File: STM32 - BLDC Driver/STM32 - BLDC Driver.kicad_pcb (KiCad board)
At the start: 2 copper layers, 15 parts, among them J1 Conn_01x02_Pin, J4 TC2050, U1 STM32F411CEUx, U2 LM2596S-3.3, U6 LD1117S33TR_SOT223, U7 LM66100DCK, U8 LM66100DCK

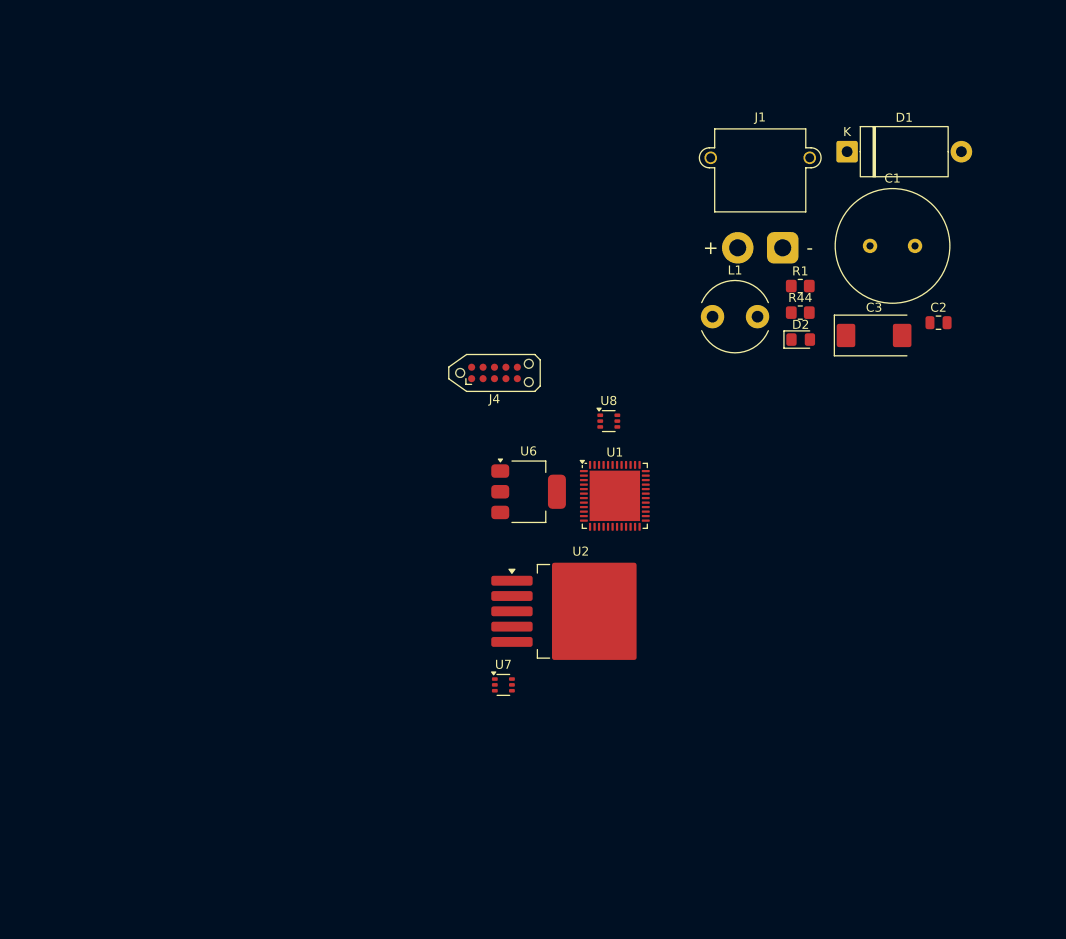
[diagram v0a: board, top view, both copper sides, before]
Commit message: As manufactured.
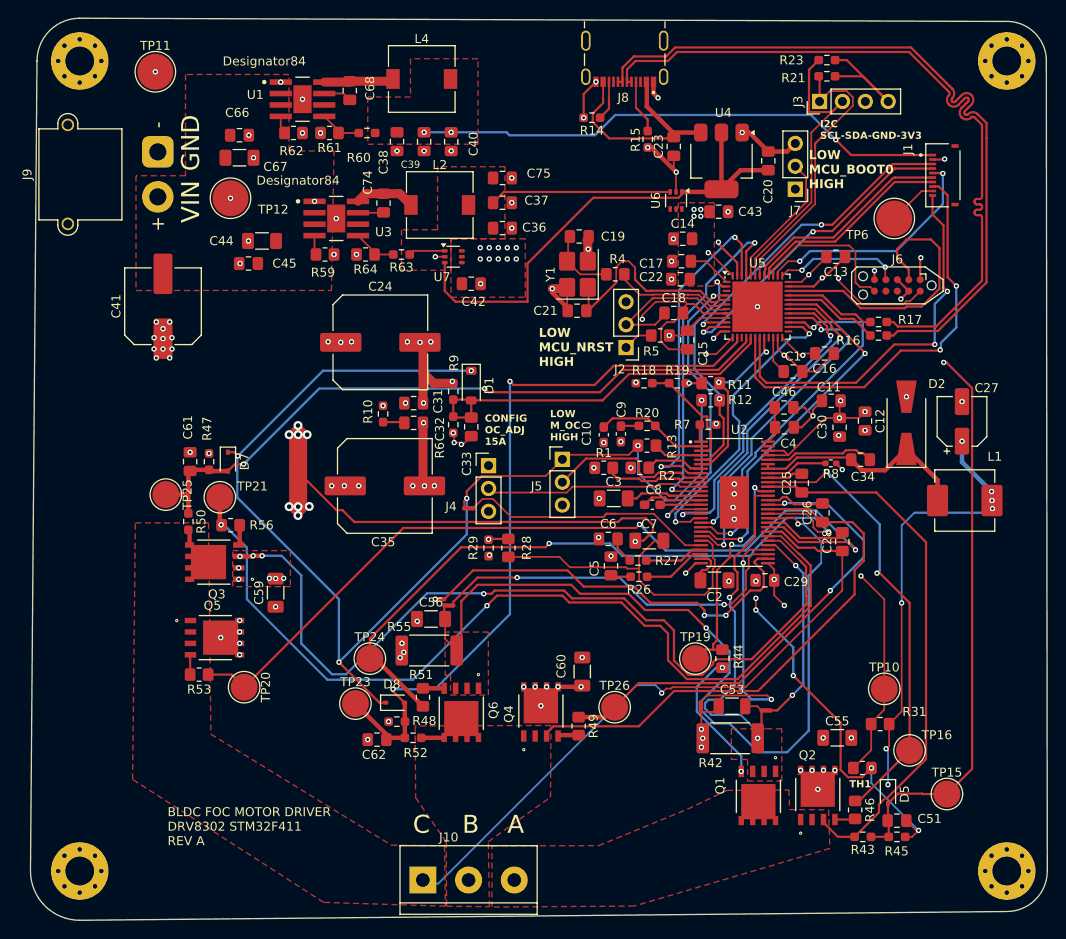
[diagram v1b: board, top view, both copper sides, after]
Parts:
- removed U8: LM66100DCK, Package_TO_SOT_SMD:SOT-363_SC-70-6
- added C10: 120p (C107035), Capacitor_SMD:C_0603_1608Metric_Pad1.08x0.95mm_HandSolder, F.Cu at (79.2, 61.5)
- added C11: 4.7u low esr (C1779), Capacitor_SMD:C_0805_2012Metric_Pad1.18x1.45mm_HandSolder, F.Cu at (104.5, 57.8)
- added C12: 4.7u low esr (C1779), Capacitor_SMD:C_0805_2012Metric_Pad1.18x1.45mm_HandSolder, F.Cu at (108.2, 60.0)
- added C13: 100nF 50V (C28233), Capacitor_SMD:C_0805_2012Metric_Pad1.18x1.45mm_HandSolder, F.Cu at (105.0, 41.8)
- added C14: 100nF 50V (C28233), Capacitor_SMD:C_0805_2012Metric_Pad1.18x1.45mm_HandSolder, F.Cu at (88.0, 39.8)
- added C15: 100nF 50V (C28233), Capacitor_SMD:C_0805_2012Metric_Pad1.18x1.45mm_HandSolder, F.Cu at (88.5, 51.0)
- added C16: 100nF 50V (C28233), Capacitor_SMD:C_0805_2012Metric_Pad1.18x1.45mm_HandSolder, F.Cu at (103.8, 52.5)
- added C17: 2.2u (C5448893), Capacitor_SMD:C_0805_2012Metric_Pad1.18x1.45mm_HandSolder, F.Cu at (87.9, 42.2)
- added C18: 100nF 50V (C28233), Capacitor_SMD:C_0805_2012Metric_Pad1.18x1.45mm_HandSolder, F.Cu at (87.0, 48.0)
- added C19: 100nF 50V (C28233), Capacitor_SMD:C_0805_2012Metric_Pad1.18x1.45mm_HandSolder, F.Cu at (76.5, 39.5)
- added C20: 10uF (C15850), Capacitor_SMD:C_0805_2012Metric_Pad1.18x1.45mm_HandSolder, F.Cu at (97.5, 31.1)
- added C21: 100nF 50V (C28233), Capacitor_SMD:C_0805_2012Metric_Pad1.18x1.45mm_HandSolder, F.Cu at (76.2, 47.8)
- added C22: 100nF 50V (C28233), Capacitor_SMD:C_0805_2012Metric_Pad1.18x1.45mm_HandSolder, F.Cu at (87.8, 44.2)
- added C23: 100nF 50V (C28233), Capacitor_SMD:C_0805_2012Metric_Pad1.18x1.45mm_HandSolder, F.Cu at (87.0, 29.5)
- added C24: 220uF (C46550422), Capacitor_SMD:C_Elec_10x10.2, F.Cu at (54.4, 51.3)
- added C25: 0.1uF (C28233), Capacitor_SMD:C_0805_2012Metric_Pad1.18x1.45mm_HandSolder, F.Cu at (101.2, 66.9)
- added C26: 0.1uF (C28233), Capacitor_SMD:C_0805_2012Metric_Pad1.18x1.45mm_HandSolder, F.Cu at (103.5, 70.2)
- added C27: 47uF_P (C18221497), Capacitor_SMD:CP_Elec_5x5.4, F.Cu at (119.0, 60.0)
- added C28: 0.1uF (C28233), Capacitor_SMD:C_0805_2012Metric_Pad1.18x1.45mm_HandSolder, F.Cu at (105.7, 73.4)
- added C29: 0.1uF (C28233), Capacitor_SMD:C_0805_2012Metric_Pad1.18x1.45mm_HandSolder, F.Cu at (97.1, 77.7)
- added C30: 0.1uF (C28233), Capacitor_SMD:C_0805_2012Metric_Pad1.18x1.45mm_HandSolder, F.Cu at (105.4, 60.7)
- added C31: 0.1uF (C28233), Capacitor_SMD:C_0805_2012Metric_Pad1.18x1.45mm_HandSolder, F.Cu at (58.1, 58.0)
- added C32: 0.01uF (C1710), Capacitor_SMD:C_0805_2012Metric_Pad1.18x1.45mm_HandSolder, F.Cu at (58.1, 60.2)
- added C33: 0.1uF (C28233), Capacitor_SMD:C_0805_2012Metric_Pad1.18x1.45mm_HandSolder, F.Cu at (64.5, 60.6)
- added C34: 0.1uF (C28233), Capacitor_SMD:C_0805_2012Metric_Pad1.18x1.45mm_HandSolder, F.Cu at (107.7, 64.3)
- added C35: 220uF (C46550422), Capacitor_SMD:C_Elec_10x10.2, F.Cu at (54.9, 67.2)
- added C36: 22uF (C45783), Capacitor_SMD:C_0805_2012Metric_Pad1.18x1.45mm_HandSolder, F.Cu at (68.0, 38.6)
- added C37: 22uF (C45783), Capacitor_SMD:C_0805_2012Metric_Pad1.18x1.45mm_HandSolder, F.Cu at (68.0, 35.8)
- added C38: 22uF (C45783), Capacitor_SMD:C_0805_2012Metric_Pad1.18x1.45mm_HandSolder, F.Cu at (56.2, 29.0)
- added C39: 22uF (C45783), Capacitor_SMD:C_0805_2012Metric_Pad1.18x1.45mm_HandSolder, F.Cu at (59.3, 29.0)
- added C4: 10nF (C1710), Capacitor_SMD:C_0805_2012Metric_Pad1.18x1.45mm_HandSolder, F.Cu at (99.3, 60.7)
- added C40: 22uF (C45783), Capacitor_SMD:C_0805_2012Metric_Pad1.18x1.45mm_HandSolder, F.Cu at (62.3, 29.0)
- added C41: 100uF 63V (C7471891), Capacitor_SMD:C_Elec_8x10.2, F.Cu at (30.2, 47.2)
- added C42: 4.7u low esr (C1779), Capacitor_SMD:C_0805_2012Metric_Pad1.18x1.45mm_HandSolder, F.Cu at (64.5, 44.8)
- added C43: 4.7u low esr (C1779), Capacitor_SMD:C_0805_2012Metric_Pad1.18x1.45mm_HandSolder, F.Cu at (92.0, 36.8)
- added C44: 4.7uF 50V (C29823), Capacitor_SMD:C_1206_3216Metric_Pad1.33x1.80mm_HandSolder, F.Cu at (41.2, 40.0)
- added C45: 100nF 50V (C28233), Capacitor_SMD:C_0805_2012Metric_Pad1.18x1.45mm_HandSolder, F.Cu at (39.8, 42.5)
- added C46: 4.7nF (C1744), Capacitor_SMD:C_0805_2012Metric_Pad1.18x1.45mm_HandSolder, F.Cu at (99.2, 58.5)
- added C5: 2.2nF (C28260), Capacitor_SMD:C_0805_2012Metric_Pad1.18x1.45mm_HandSolder, F.Cu at (80.0, 76.1)
- added C51: 0.1uF (C28233), Capacitor_SMD:C_0805_2012Metric_Pad1.18x1.45mm_HandSolder, F.Cu at (111.8, 104.4)
- added C53: 1nF (C9196), Capacitor_SMD:C_1206_3216Metric, F.Cu at (93.5, 91.7)
- added C55: 2.2uF (C50254), Capacitor_SMD:C_1206_3216Metric_Pad1.33x1.80mm_HandSolder, F.Cu at (105.2, 95.2)
- added C56: 1nF (C9196), Capacitor_SMD:C_1206_3216Metric_Pad1.33x1.80mm_HandSolder, F.Cu at (60.0, 82.0)
- added C59: 2.2uF (C50254), Capacitor_SMD:C_1206_3216Metric_Pad1.33x1.80mm_HandSolder, F.Cu at (42.8, 79.1)
- added C6: 2.2nF (C28260), Capacitor_SMD:C_0805_2012Metric_Pad1.18x1.45mm_HandSolder, F.Cu at (79.7, 73.1)
- added C60: 2.2uF (C50254), Capacitor_SMD:C_1206_3216Metric_Pad1.33x1.80mm_HandSolder, F.Cu at (76.8, 87.8)
- added C61: 0.1uF (C28233), Capacitor_SMD:C_0805_2012Metric_Pad1.18x1.45mm_HandSolder, F.Cu at (33.3, 64.5)
- added C62: 0.1uF (C28233), Capacitor_SMD:C_0805_2012Metric_Pad1.18x1.45mm_HandSolder, F.Cu at (54.0, 95.4)
- added C66: 100nF 50V (C28233), Capacitor_SMD:C_0805_2012Metric_Pad1.18x1.45mm_HandSolder, F.Cu at (38.8, 28.2)
- added C67: 4.7uF 50V (C29823), Capacitor_SMD:C_1206_3216Metric_Pad1.33x1.80mm_HandSolder, F.Cu at (38.8, 30.8)
- added C68: 0.1uF (C28233), Capacitor_SMD:C_0805_2012Metric_Pad1.18x1.45mm_HandSolder, F.Cu at (51.0, 23.3)
- added C7: 1uF (C13832), Capacitor_SMD:C_1206_3216Metric_Pad1.33x1.80mm_HandSolder, F.Cu at (84.3, 73.3)
- added C74: 0.1uF (C28233), Capacitor_SMD:C_0805_2012Metric_Pad1.18x1.45mm_HandSolder, F.Cu at (54.8, 35.8)
- added C75: 22uF (C45783), Capacitor_SMD:C_0805_2012Metric_Pad1.18x1.45mm_HandSolder, F.Cu at (68.0, 33.0)
- added C8: 22nF (C376821), Capacitor_SMD:C_0603_1608Metric_Pad1.08x0.95mm_HandSolder, F.Cu at (84.6, 69.3)
- added C9: 6.8n (C1631), Capacitor_SMD:C_0603_1608Metric_Pad1.08x0.95mm_HandSolder, F.Cu at (81.1, 61.4)
- added D5: D_Zener (C67528), Diode_SMD:D_SOD-323, F.Cu at (110.8, 101.5)
- added D7: D_Zener (C67528), Diode_SMD:D_SOD-323, F.Cu at (37.5, 64.5)
- added D8: D_Zener (C67528), Diode_SMD:D_SOD-323, F.Cu at (56.0, 91.3)
- added H1: MountingHole_Pad, MountingHole:MountingHole_3.2mm_M3_Pad_Via, F.Cu at (124.0, 110.0)
- added H2: MountingHole_Pad, MountingHole:MountingHole_3.2mm_M3_Pad_Via, F.Cu at (124.0, 20.0)
- added H3: MountingHole_Pad, MountingHole:MountingHole_3.2mm_M3_Pad_Via, F.Cu at (21.0, 110.0)
- added H4: MountingHole_Pad, MountingHole:MountingHole_3.2mm_M3_Pad_Via, F.Cu at (21.0, 20.0)
- added J10: Screw_Terminal_01x03, TerminalBlock:TerminalBlock_bornier-3_P5.08mm, F.Cu at (59.1, 111.0)
- added J2: Conn_01x03_Pin, Connector_PinHeader_2.54mm:PinHeader_1x03_P2.54mm_Vertical, F.Cu at (81.7, 51.8)
- added J3: Conn_01x04_Pin, Connector_PinHeader_2.54mm:PinHeader_1x04_P2.54mm_Vertical, F.Cu at (103.2, 24.5)
- added J5: Conn_01x03_Pin, Connector_PinHeader_2.54mm:PinHeader_1x03_P2.54mm_Vertical, F.Cu at (74.6, 64.3)
- added J6: TC2050, Connector:Tag-Connect_TC2050-IDC-NL_2x05_P1.27mm_Vertical, F.Cu at (111.8, 44.9)
- added J7: Conn_01x03_Pin, Connector_PinHeader_2.54mm:PinHeader_1x03_P2.54mm_Vertical, F.Cu at (100.5, 34.2)
- added J8: GT-USB-7010B, GT-USB-7010B:G-SWITCH_GT-USB-7010B, F.Cu at (81.5, 17.8)
- added J9: Conn_01x02_Pin, Connector_AMASS:AMASS_XT30PW-M_1x02_P2.50mm_Horizontal, F.Cu at (29.7, 30.1)
- added L2: 15uH (C216196), Inductor_SMD:L_7.3x7.3_H3.5, F.Cu at (61.0, 36.0)
- added L4: 15uH (C216196), Inductor_SMD:L_7.3x7.3_H3.5, F.Cu at (59.0, 22.0)
- added NT1: NetTie_3_Tee, NetTie:NetTie-3_SMD_Pad2.0mm, F.Cu at (45.3, 65.5)
- added NT2: NetTie_2, NetTie:NetTie-2_SMD_Pad0.5mm, F.Cu at (40.8, 75.0)
- added NT3: NetTie_2, NetTie:NetTie-2_SMD_Pad0.5mm, F.Cu at (90.0, 91.8)
- added NT4: NetTie_2, NetTie:NetTie-2_SMD_Pad0.5mm, F.Cu at (61.0, 79.8)
- added NT5: NetTie_2, NetTie:NetTie-2_SMD_Pad0.5mm, F.Cu at (64.2, 69.7)
- added NT6: NetTie_2, NetTie:NetTie-2_SMD_Pad0.5mm, F.Cu at (62.0, 80.5)
- added NT8: NetTie_2, NetTie:NetTie-2_SMD_Pad0.5mm, F.Cu at (97.2, 92.2)
- added Q1: SIR182DP-T1-RE3, SIR182DP:TRANS_SIR182DP-T1-RE3, F.Cu at (96.4, 101.6)
- added Q2: SIR182DP-T1-RE3, SIR182DP:TRANS_SIR182DP-T1-RE3, F.Cu at (103.0, 101.6)
- added Q3: SIR182DP-T1-RE3, SIR182DP:TRANS_SIR182DP-T1-RE3, F.Cu at (36.0, 75.7)
- added Q4: SIR182DP-T1-RE3, SIR182DP:TRANS_SIR182DP-T1-RE3, F.Cu at (72.2, 92.3)
- added Q5: SIR182DP-T1-RE3, SIR182DP:TRANS_SIR182DP-T1-RE3, F.Cu at (36.0, 84.1)
- added Q6: SIR182DP-T1-RE3, SIR182DP:TRANS_SIR182DP-T1-RE3, F.Cu at (63.4, 92.4)
- added R10: 3.3R (C22979), Resistor_SMD:R_0603_1608Metric_Pad0.98x0.95mm_HandSolder, F.Cu at (54.7, 59.2)
- added R11: 10k (C17414), Resistor_SMD:R_0805_2012Metric_Pad1.20x1.40mm_HandSolder, F.Cu at (91.1, 55.8)
- added R12: 10k (C17414), Resistor_SMD:R_0805_2012Metric_Pad1.20x1.40mm_HandSolder, F.Cu at (91.1, 57.7)
- added R13: 10k (C17414), Resistor_SMD:R_0805_2012Metric_Pad1.20x1.40mm_HandSolder, F.Cu at (84.0, 62.7)
- added R14: 5.1k (C22356620), Resistor_SMD:R_0603_1608Metric_Pad0.98x0.95mm_HandSolder, F.Cu at (77.9, 26.3)
- added R15: 5.1k (C22356620), Resistor_SMD:R_0603_1608Metric_Pad0.98x0.95mm_HandSolder, F.Cu at (84.1, 28.7)
- added R16: 0R, Resistor_SMD:R_0603_1608Metric_Pad0.98x0.95mm_HandSolder, F.Cu at (109.8, 50.5)
- added R17: 0R, Resistor_SMD:R_0603_1608Metric_Pad0.98x0.95mm_HandSolder, F.Cu at (109.8, 49.0)
- added R18: 3k3 (C22356670), Resistor_SMD:R_0603_1608Metric_Pad0.98x0.95mm_HandSolder, F.Cu at (83.7, 55.8)
- added R19: 18k (C2907111), Resistor_SMD:R_0603_1608Metric_Pad0.98x0.95mm_HandSolder, F.Cu at (87.4, 55.8)
- added R2: 10k (C17414), Resistor_SMD:R_0805_2012Metric_Pad1.20x1.40mm_HandSolder, F.Cu at (83.2, 65.2)
- added R20: 15k (C22356635), Resistor_SMD:R_0603_1608Metric_Pad0.98x0.95mm_HandSolder, F.Cu at (84.0, 60.5)
- added R21: 2.2k (C4190), Resistor_SMD:R_0603_1608Metric_Pad0.98x0.95mm_HandSolder, F.Cu at (104.0, 21.7)
- added R23: 2.2k (C4190), Resistor_SMD:R_0603_1608Metric_Pad0.98x0.95mm_HandSolder, F.Cu at (104.0, 19.9)
- added R26: 56R (C2930118), Resistor_SMD:R_0603_1608Metric_Pad0.98x0.95mm_HandSolder, F.Cu at (83.1, 77.3)
- added R27: 56R (C2930118), Resistor_SMD:R_0603_1608Metric_Pad0.98x0.95mm_HandSolder, F.Cu at (83.0, 75.5)
- added R28: 1k (C22356624), Resistor_SMD:R_0603_1608Metric_Pad0.98x0.95mm_HandSolder, F.Cu at (66.4, 74.1)
- added R29: 80.6k (C2960781), Resistor_SMD:R_0805_2012Metric_Pad1.20x1.40mm_HandSolder, F.Cu at (68.6, 74.1)
- added R31: 8.2k (C17828), Resistor_SMD:R_0805_2012Metric_Pad1.20x1.40mm_HandSolder, F.Cu at (109.9, 93.7)
- added R4: 0R (C17477), Resistor_SMD:R_0805_2012Metric_Pad1.20x1.40mm_HandSolder, F.Cu at (80.5, 43.7)
- added R42: 10mOhm (C393072), Resistor_SMD:R_2512_6332Metric_Pad1.40x3.35mm_HandSolder, F.Cu at (93.3, 95.2)
- added R43: 34.8k (C23141), Resistor_SMD:R_0603_1608Metric_Pad0.98x0.95mm_HandSolder, F.Cu at (108.0, 106.2)
- added R45: 4.99k (C23046), Resistor_SMD:R_0603_1608Metric_Pad0.98x0.95mm_HandSolder, F.Cu at (111.8, 106.2)
- added R46: 10R (C17415), Resistor_SMD:R_0805_2012Metric_Pad1.20x1.40mm_HandSolder, F.Cu at (107.2, 103.2)
- added R47: 4.99k (C23046), Resistor_SMD:R_0603_1608Metric_Pad0.98x0.95mm_HandSolder, F.Cu at (35.4, 64.5)
- added R48: 4.99k (C23046), Resistor_SMD:R_0603_1608Metric_Pad0.98x0.95mm_HandSolder, F.Cu at (56.2, 93.4)
- added R49: 10R (C17415), Resistor_SMD:R_0805_2012Metric_Pad1.20x1.40mm_HandSolder, F.Cu at (76.4, 93.9)
- added R5: 10k (C17414), Resistor_SMD:R_0805_2012Metric_Pad1.20x1.40mm_HandSolder, F.Cu at (85.5, 50.5)
- added R50: 34.8k (C23141), Resistor_SMD:R_0603_1608Metric_Pad0.98x0.95mm_HandSolder, F.Cu at (33.1, 71.2)
- added R51: 10R (C17415), Resistor_SMD:R_0805_2012Metric_Pad1.20x1.40mm_HandSolder, F.Cu at (59.1, 90.7)
- added R52: 34.8k (C23141), Resistor_SMD:R_0603_1608Metric_Pad0.98x0.95mm_HandSolder, F.Cu at (58.0, 95.2)
- added R53: 10R (C17415), Resistor_SMD:R_0805_2012Metric_Pad1.20x1.40mm_HandSolder, F.Cu at (34.3, 88.2)
- added R55: 10mOhm (C393072), Resistor_SMD:R_2512_6332Metric_Pad1.40x3.35mm_HandSolder, F.Cu at (59.8, 85.5)
- added R56: 10R (C17415), Resistor_SMD:R_0805_2012Metric_Pad1.20x1.40mm_HandSolder, F.Cu at (37.8, 71.6)
- added R59: 64.9k (C17788), Resistor_SMD:R_0805_2012Metric_Pad1.20x1.40mm_HandSolder, F.Cu at (48.2, 41.5)
- added R6: 4.99k (C23046), Resistor_SMD:R_0603_1608Metric_Pad0.98x0.95mm_HandSolder, F.Cu at (62.5, 60.4)
- added R60: 100k (C15458), Resistor_SMD:R_0603_1608Metric_Pad0.98x0.95mm_HandSolder, F.Cu at (52.9, 28.0)
- added R61: 24.9k (C17571), Resistor_SMD:R_0805_2012Metric_Pad1.20x1.40mm_HandSolder, F.Cu at (48.8, 28.0)
- added R62: 64.9k (C17788), Resistor_SMD:R_0805_2012Metric_Pad1.20x1.40mm_HandSolder, F.Cu at (44.8, 28.0)
- added R63: 57.6k (C204216), Resistor_SMD:R_0603_1608Metric_Pad0.98x0.95mm_HandSolder, F.Cu at (56.8, 41.5)
- added R64: 24.9k (C17571), Resistor_SMD:R_0805_2012Metric_Pad1.20x1.40mm_HandSolder, F.Cu at (52.8, 41.5)
- added R7: 200k (C25811), Resistor_SMD:R_0603_1608Metric_Pad0.98x0.95mm_HandSolder, F.Cu at (90.8, 60.4)
- added R8: 1M (C26083), Resistor_SMD:R_0402_1005Metric_Pad0.72x0.64mm_HandSolder, F.Cu at (104.4, 64.7)
- added R9: 34.8k (C23141), Resistor_SMD:R_0603_1608Metric_Pad0.98x0.95mm_HandSolder, F.Cu at (62.5, 56.7)
- added TH1: CMFB103F3950FANT (C51597), Resistor_SMD:R_0805_2012Metric_Pad1.20x1.40mm_HandSolder, F.Cu at (108.0, 98.6)
- added TP10: TestPoint, TestPoint:TestPoint_Pad_D3.0mm, F.Cu at (110.4, 89.8)
- added TP11: TestPoint, TestPoint:TestPoint_Pad_D4.0mm, F.Cu at (29.4, 21.2)
- added TP12: TestPoint, TestPoint:TestPoint_Pad_D4.0mm, F.Cu at (37.8, 35.2)
- added TP15: TestPoint, TestPoint:TestPoint_Pad_D3.0mm, F.Cu at (117.3, 101.4)
- added TP16: TestPoint, TestPoint:TestPoint_Pad_D3.0mm, F.Cu at (113.2, 96.6)
- added TP19: TestPoint, TestPoint:TestPoint_Pad_D3.0mm, F.Cu at (89.4, 86.4)
- added TP20: TestPoint, TestPoint:TestPoint_Pad_D3.0mm, F.Cu at (39.3, 89.6)
- added TP21: TestPoint, TestPoint:TestPoint_Pad_D3.0mm, F.Cu at (36.6, 68.5)
- added TP23: TestPoint, TestPoint:TestPoint_Pad_D3.0mm, F.Cu at (51.6, 91.4)
- added TP24: TestPoint, TestPoint:TestPoint_Pad_D3.0mm, F.Cu at (53.2, 86.4)
- added TP25: TestPoint, TestPoint:TestPoint_Pad_D3.0mm, F.Cu at (30.6, 68.2)
- added TP26: TestPoint, TestPoint:TestPoint_Pad_D3.0mm, F.Cu at (80.4, 91.8)
- added TP6: TestPoint, TestPoint:TestPoint_Pad_D4.0mm, F.Cu at (111.5, 37.5)
- added U3: LMR38020SDDAR, LMR38020SDDAR:DDA0008E-IPC_A, F.Cu at (49.5, 37.5)
- added U4: LD1117S33TR_SOT223, Package_TO_SOT_SMD:SOT-223-3_TabPin2, F.Cu at (92.3, 31.1)
- added U5: STM32F411CEUx, Package_DFN_QFN:QFN-48-1EP_7x7mm_P0.5mm_EP5.6x5.6mm, F.Cu at (96.3, 47.3)
- added Y1: Crystal_GND24 (C5444547), Crystal:Crystal_SMD_3225-4Pin_3.2x2.5mm_HandSoldering, F.Cu at (76.3, 43.7)
- C1: value 680uF LOW ESR ( C443017 ) -> 4.7u low esr (C1779); footprint Capacitor_THT:C_Radial_D12.5mm_H20.0mm_P5.00mm -> Capacitor_SMD:C_0805_2012Metric_Pad1.18x1.45mm_HandSolder
- C2: value 0.1uF Ceramic (CL21B104KBCNNNC ) -> 1uF (C13832); footprint Capacitor_SMD:C_0805_2012Metric -> Capacitor_SMD:C_1206_3216Metric_Pad1.33x1.80mm_HandSolder
- C3: value C600568 -> 2.2uF (C920964); footprint Capacitor_Tantalum_SMD:CP_EIA-7343-43_Kemet-X -> Capacitor_SMD:C_1206_3216Metric_Pad1.33x1.80mm_HandSolder
- D1: value SR502 (HandSoldered) -> D_Zener (C173406); footprint Diode_THT:D_DO-27_P12.70mm_Horizontal -> Diode_SMD:D_SOD-123
- D2: value C2297 -> B330A-13-F (C110485); footprint LED_SMD:LED_0805_2012Metric_Pad1.15x1.40mm_HandSolder -> Diode_SMD:D_SMA-SMB_Universal_Handsoldering
- J1: value Conn_01x02_Pin -> FH34SRJ-10S-0.5SH_50_; footprint Connector_AMASS:AMASS_XT30PW-M_1x02_P2.50mm_Horizontal -> FH34SRJ-10S-0.5SH:HRS_FH34SRJ-10S-0.5SH_50_
- J4: value TC2050 -> Conn_01x03_Pin; footprint Connector:Tag-Connect_TC2050-IDC-NL_2x05_P1.27mm_Vertical -> Connector_PinHeader_2.54mm:PinHeader_1x03_P2.54mm_Vertical
- L1: value 7447720330 (HandSolder) -> 22uH (C177244); footprint Inductor_THT:L_Radial_D7.8mm_P5.00mm_Fastron_07HCP -> Inductor_SMD:L_Changjiang_FXL0630
- R1: value 5Ohm (C17724) -> 10k (C17414)
- R44: value 5kOhm (C2073749) -> 10R (C17415)
- U1: value STM32F411CEUx -> LMR38020SDDAR; footprint Package_DFN_QFN:QFN-48-1EP_7x7mm_P0.5mm_EP5.6x5.6mm -> LMR38020SDDAR:DDA0008E-IPC_A
- U2: value LM2596S-3.3 -> DRV8302DCAR; footprint Package_TO_SOT_SMD:TO-263-5_TabPin3 -> DRV8302DCAR:SOP50P810X120-57N
- U6: value LD1117S33TR_SOT223 -> LM66100DCK; footprint Package_TO_SOT_SMD:SOT-223-3_TabPin2 -> Package_TO_SOT_SMD:SOT-363_SC-70-6
- moved U1 56.1 mm to (45.8, 24.2)
- moved D1 49.2 mm to (64.5, 56.1), turned to -90 degrees
- moved U7 47.9 mm to (62.5, 41.8)
- moved R44 39.4 mm to (92.4, 86.4), turned to 90 degrees
- moved C2 37.9 mm to (91.5, 77.7), turned to 180 degrees
- moved U6 36.3 mm to (87.2, 35.5), turned to -90 degrees
- moved L1 34.7 mm to (119.3, 68.8)
- moved C3 34.1 mm to (80.3, 68.6)
- moved R1 29.7 mm to (79.2, 65.2)
- moved U2 20.9 mm to (93.7, 69.0)
- moved J1 19.5 mm to (116.9, 32.7), turned to 90 degrees
- moved C1 16.4 mm to (100.2, 54.5)
- moved D2 15.0 mm to (112.8, 60.2), turned to 90 degrees
- moved J4 10.3 mm to (66.4, 65.0)
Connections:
- C1 pad 1: +24V -> /STM32G/MCU_VCAP1
- C1 pad 2: AGND -> GND
- C2 pad 1: +24V -> AGND
- C2 pad 2: AGND -> Net-(U2-AVDD)
- C3 pad 1: Net-(U2-FB) -> GND
- C3 pad 2: AGND -> Net-(U2-GVDD)
- D1 pad 1: Net-(D1-K) -> +3V3
- D1 pad 2: AGND -> PVDDSENSE
- D2 pad 1: AGND -> Net-(D2-K)
- D2 pad 2: Net-(D2-A) -> GND
- J1 pad 1: AGND -> 5V
- J1 pad 2: +24V -> GND
- J4 pad 1: DRV8302_REF -> unconnected-(J4-Pin_1-Pad1)
- J4 pad 2: MCU_SWDIO -> /DRV8302DCAR/OC_ADJ
- J4 pad 3: AGND -> Net-(J4-Pin_3)
- L1 pad 1: Net-(D1-K) -> Net-(D2-K)
- L1 pad 2: Net-(U2-FB) -> +3V3
- R1 pad 1: Net-(D2-A) -> GND
- R1 pad 2: Net-(U2-FB) -> GAIN
- R44 pad 1: DRV8302_REF -> Net-(Q1-Pad4)
- R44 pad 2: Net-(U7-ST) -> GL_A
- U1 pad 1: DRV8302_REF -> GND
- U1 pad 2: nOCTW -> PVDD
- U1 pad 3: AS5600_OUT -> PVDD
- U1 pad 4: EN_GATE -> Net-(U1-RT_SYNC)
- U1 pad 5: /STM32G/MCU_OSC_IN -> Net-(U1-FB)
- U1 pad 6: /STM32G/MCU_OSC_OUT -> unconnected-(U1-PG-Pad6)
- U1 pad 7: MCU_NRST -> Net-(U1-BOOT)
- U1 pad 8: AGND -> Net-(U1-SW)
- U1 pad 9: DRV8302_REF -> GND
- U2 pad 1: +24V -> /DRV8302DCAR/DRV_RC_CLK
- U2 pad 2: Net-(D1-K) -> /DRV8302DCAR/DRV_COMP
- U2 pad 3: AGND -> Net-(U2-VSENSE)
- U2 pad 4: Net-(U2-FB) -> DRV_PWRGD
- U2 pad 5: AGND -> nOCTW
- U6 pad 1: AGND -> USB_3V3
- U6 pad 2: Net-(U6-VO) -> GND
- U6 pad 3: USB_VBUS -> MAIN_3V3
- U7 pad 1: Net-(U2-FB) -> MAIN_3V3
- U7 pad 2: AGND -> GND
- U7 pad 3: DRV8302_REF -> USB_3V3
- U7 pad 5: Net-(U7-ST) -> unconnected-(U7-ST-Pad5)
- U7 pad 6: DRV8302_REF -> +3V3
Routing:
- net GND: track 0.00 -> 587.2 mm, vias 0 -> 89
- net +3V3: track 0.00 -> 225.7 mm, vias 0 -> 33
- net GL_C: track 0.00 -> 102.6 mm, vias 0 -> 2
- net GH_C: track 0.00 -> 95.7 mm, vias 0 -> 2
- net SL_B: track 0.00 -> 95.4 mm, vias 0 -> 2
- net SL_C: track 0.00 -> 93.1 mm, vias 0 -> 2
- net ASENSE: track 0.00 -> 91.8 mm, vias 0 -> 2
- net BSENSE: track 0.00 -> 83.7 mm, vias 0 -> 2
- net /STM32G/D-: track 0.00 -> 82.3 mm
- net /STM32G/D+: track 0.00 -> 82.3 mm
- net GL_B: track 0.00 -> 76.7 mm, vias 0 -> 2
- net SH_C: track 0.00 -> 76.5 mm, vias 0 -> 1
- net CSENSE: track 0.00 -> 76.1 mm, vias 0 -> 2
- net MOS1_NTC: track 0.00 -> 70.8 mm, vias 0 -> 2
- net SH_B: track 0.00 -> 62.4 mm
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- added copper zone on F.Cu, net +3V3
- added copper zone on In2.Cu, net +3V3
- added copper zone on F.Cu, net 5V
- added copper zone on In1.Cu, net GND
- added copper zone on F.Cu, net MAIN_3V3
- added copper zone on F.Cu, net PGND
- added copper zone on In1.Cu, net PGND
- added copper zone on F.Cu, net PVDD
- added copper zone on In2.Cu, net PVDD
- added copper zone on F.Cu, net SH_A
- added copper zone on F.Cu, net SH_B
- added copper zone on F.Cu, net SH_C
- added copper zone on F.Cu, net SL_A
- added copper zone on F.Cu, net SL_B
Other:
- board outline added: 113 x 100.2 mm
- copper layers 2 -> 4
- board text added: "A"
- board text added: "B"
- board text added: "BLDC FOC MOTOR DRIVER DRV8302 STM32F411 REV A"
- board text added: "C"
- board text added: "CONFIG OC_ADJ 15A"
- board text added: "GND"
- board text added: "I2C SCL-SDA-GND-3V3"
- board text added: "LOW MCU_BOOT0 HIGH"
- board text added: "LOW MCU_NRST HIGH"
- board text added: "LOW M_OC HIGH"
- board text added: "VIN"
